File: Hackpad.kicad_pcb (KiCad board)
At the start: 2 copper layers, 85 x 90.5 mm, 21 parts, among them SW1 SW_Push, SW10 RotaryEncoder_Switch, SW2 SW_Push, SW3 SW_Push, SW4 SW_Push, SW5 SW_Push, SW6 SW_Push, SW7 SW_Push, SW8 SW_Push, SW9 SW_Push, U1 MOUDLE-SEEEDUINO-XIAO, U2 ER_OLEDM0.91_1x-I2C

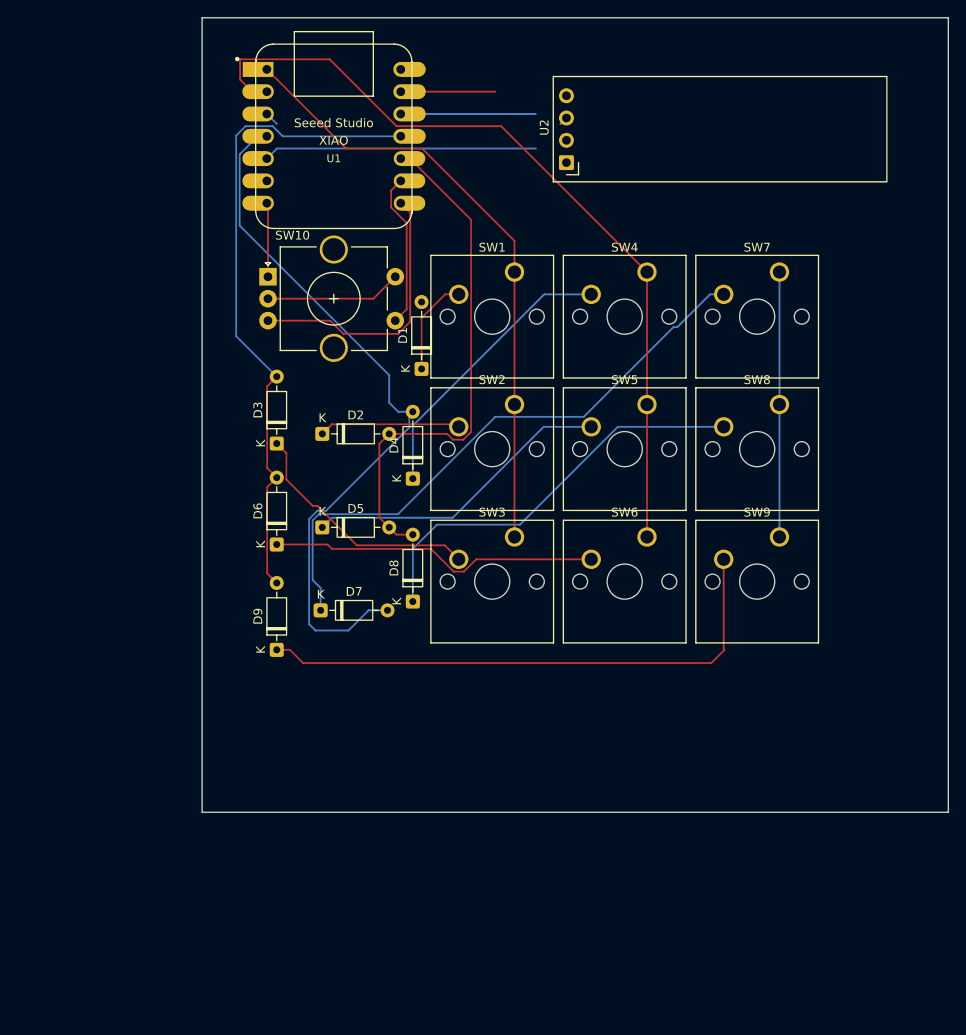
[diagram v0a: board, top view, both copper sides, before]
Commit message: ain
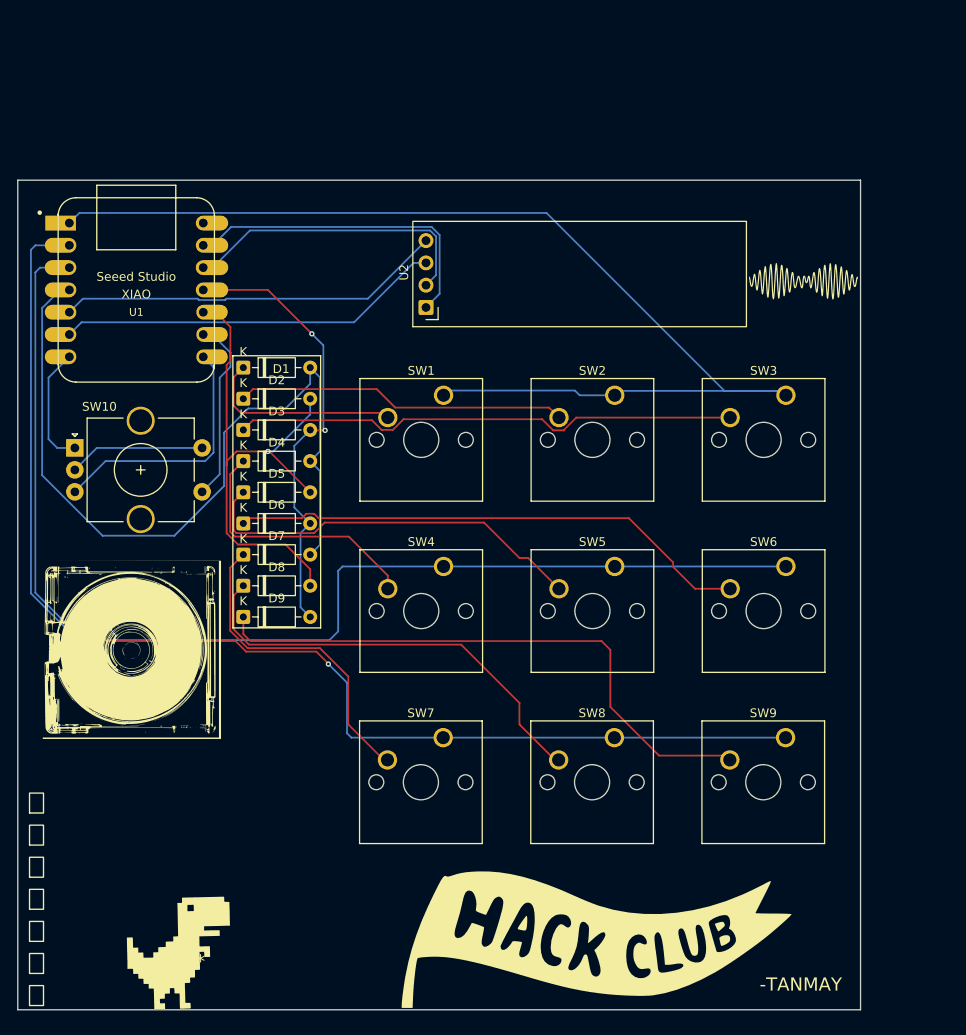
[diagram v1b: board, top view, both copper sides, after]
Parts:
- added G***: LOGO, LOGO, F.Cu at (146.5, 59.5)
- added G***: LOGO, LOGO, F.Cu at (123.0, 134.5)
- added G***: LOGO, LOGO, F.Cu at (70.0, 101.5)
- added G***: LOGO, LOGO, F.Cu at (76.0, 137.0)
- added G***: LOGO, LOGO, B.Cu at (87.0, 120.0)
- added G***: LOGO, LOGO, B.Cu at (126.0, 109.5)
- added G***: LOGO, LOGO, B.Cu at (112.5, 81.0)
- moved SW7 65.4 mm to (105.5, 111.5)
- moved SW8 42.3 mm to (125.0, 111.5)
- moved SW4 40.8 mm to (105.5, 92.0)
- moved SW3 34.9 mm to (144.5, 72.5)
- moved SW10 29.4 mm to (63.5, 78.5)
- moved U1 28.5 mm to (70.5, 60.5)
- moved U2 23.0 mm to (103.5, 62.5)
- moved SW9 22.9 mm to (144.5, 111.5)
- moved D1 20.3 mm to (82.7, 69.3), turned to 0 degrees
- moved D4 19.4 mm to (82.7, 80.0), turned to 0 degrees
- moved D8 19.4 mm to (82.7, 94.2), turned to 0 degrees
- moved SW5 18.8 mm to (125.0, 92.0)
- moved SW1 16.2 mm to (105.5, 72.5)
- moved SW6 16.2 mm to (144.5, 92.0)
- moved SW2 11.5 mm to (125.0, 72.5)
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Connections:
- SW7 pad 1: /OLED -> /R3
- SW8 pad 1: /OLED -> /R3
- SW9 pad 1: /OLED -> /R3
- U1 pad 3: /OLED -> /R3
- U1 pad 5: /OLED -> /OLED_SDA
- U1 pad 6: /OLED -> Net-(U1-PA9_A5_D5_SCL)
- U2 pad 3: /OLED -> Net-(U1-PA9_A5_D5_SCL)
- U2 pad 4: /OLED -> /OLED_SDA
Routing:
- net /R3: track 0.00 -> 136.6 mm, vias 0 -> 2
- net /OLED: track 63.9 -> 0.00 mm
- net /R1: track 70.0 -> 129.9 mm
- net /R2: track 92.5 -> 140.0 mm
- net /OLED_SDA: track 0.00 -> 44.1 mm
- net Net-(U1-PA9_A5_D5_SCL): track 0.00 -> 44.0 mm
- net Net-(D7-K): track 68.1 -> 36.5 mm
- net Net-(D3-K): track 28.0 -> 58.7 mm
- net Net-(U1-GND): track 10.8 -> 37.1 mm
- net /C3: track 74.4 -> 51.6 mm, vias 0 -> 2
- net Net-(D6-K): track 37.7 -> 59.7 mm
- net Net-(D2-K): track 16.1 -> 37.8 mm
- net Net-(U1-3V3): track 15.4 -> 34.6 mm
- net Net-(D1-K): track 11.2 -> 22.9 mm
- net Net-(D5-K): track 35.4 -> 45.6 mm
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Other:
- board size 85 x 90.5 mm -> 96 x 94.5 mm
- board text added: "-TANMAY"
- board text added: "同 じ 星 空 の 下 で"
